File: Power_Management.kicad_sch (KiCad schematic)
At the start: 17 parts, among them J8 PWR_SRC_JMP, Q2 MOSFET_SI2333DDS-T1-BE3, U3 SN74LVC1G07DBVR

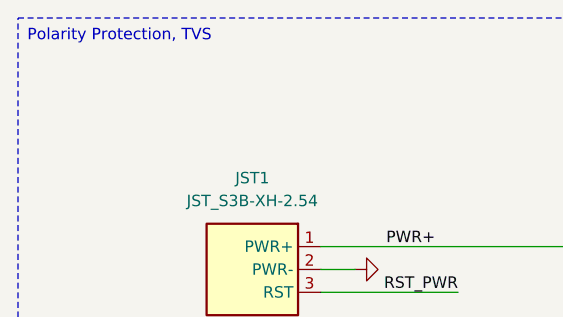
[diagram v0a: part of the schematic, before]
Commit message: Update
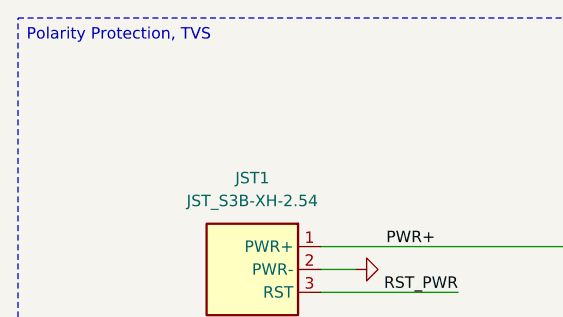
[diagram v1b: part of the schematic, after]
